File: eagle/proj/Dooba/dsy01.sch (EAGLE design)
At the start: 75 parts, among them P1 DIO, P10 SWD_CORE(SWCLK-SWDIO-GND), P11 SWD_CORE(SWCLK-SWDIO-GND), P2 CKI-CKO, P3 NOT, P4 RDY, P5 PWR(VIN-GND-RST), P6 SWD_CORE(SWCLK-SWDIO-GND), P7 SWD_CORE(SWCLK-SWDIO-GND), P8 SWD_CORE(SWCLK-SWDIO-GND), P9 SWD_CORE(SWCLK-SWDIO-GND), U1 STM32F071LQFP100, U10 S25FLXXXSSOIC16, U2 AS6C1608TSOPII-44, U3 STM32F030LQFP32, U5 STM32F030LQFP32, U6 STM32F030LQFP32, U7 STM32F030LQFP32, U8 MIC550XSOT23, U9 STM32F030LQFP32, X1 8MHz, X2 8MHz, X4 8MHz, X5 8MHz, X6 8MHz, X7 8MHz

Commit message: Finished routing DSY01 Added LEDs on DSY01
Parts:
- added D1, D2, D3, D4, D5, D6: LED0805, dooba:LED0805
- added R1, R2, R3, R4, R5, R6: 330, dooba:RES0805
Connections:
- new net N$109: R5.2, U9.PA15
- new net N$110: D6.1, R6.1
- new net N$111: R6.2, U1.PF9
- new net N$54: D1.1, R1.1
- new net N$56: R1.2, U3.PA15
- new net N$62: D2.1, R2.1
- new net N$70: R2.2, U5.PA15
- new net N$74: D3.1, R3.1
- new net N$87: R3.2, U6.PA15
- new net N$88: D4.1, R4.1
- new net N$89: R4.2, U7.PA15
- new net N$92: D5.1, R5.1
- net GND: now also D1.2, D2.2, D3.2, D4.2, D5.2, D6.2; no longer U1.PF9, U3.PA15, U5.PA15, U6.PA15, U7.PA15, U9.PA15

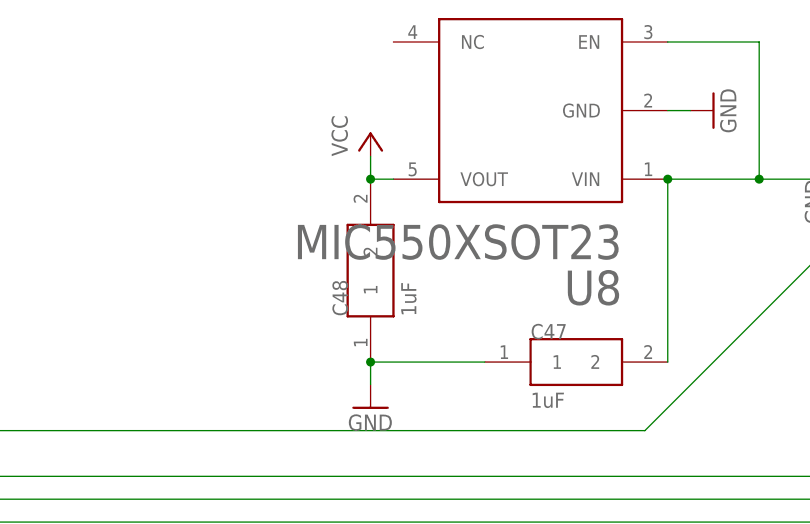
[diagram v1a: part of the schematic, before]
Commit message: Added more decorations to DSY01
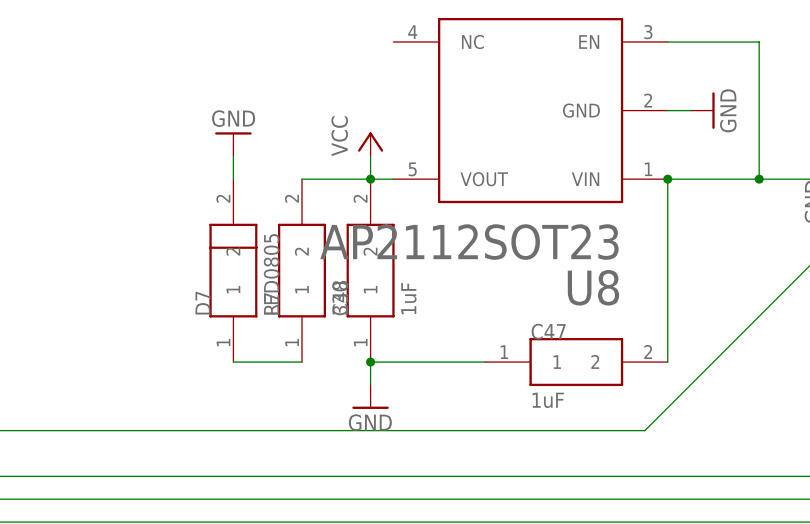
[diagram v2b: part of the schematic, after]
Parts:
- added D7: LED0805, dooba:LED0805
- added R7: 330, dooba:RES0805
- U8: value MIC550XSOT23 -> AP2112SOT23; device dooba:MIC550XSOT23 -> dooba:AP2112SOT23
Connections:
- new net N$112: D7.1, R7.1
- net GND: now also D7.2
- net VCC: now also R7.2
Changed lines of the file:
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@@
 <part name="C46" library="dooba" deviceset="CAP" device="0805" value="27pF"/>
 <part name="GND37" library="supply1" deviceset="GND" device=""/>
-<part name="U8" library="dooba" deviceset="MIC550X" device="SOT23"/>
+<part name="U8" library="dooba" deviceset="AP2112" device="SOT23"/>
 <part name="C47" library="dooba" deviceset="CAP" device="0805" value="1uF"/>
 <part name="C48" library="dooba" deviceset="CAP" device="0805" value="1uF"/>
@@
 <part name="R6" library="dooba" deviceset="RES" device="0805" value="330"/>
 <part name="GND49" library="supply1" deviceset="GND" device=""/>
+<part name="D7" library="dooba" deviceset="LED" device="0805"/>
+<part name="R7" library="dooba" deviceset="RES" device="0805" value="330"/>
+<part name="GND61" library="supply1" deviceset="GND" device=""/>
 </parts>
 <sheets>
@@
 <instance part="R6" gate="R1" x="381" y="416.56"/>
 <instance part="GND49" gate="1" x="396.24" y="424.18" rot="R90"/>
+<instance part="D7" gate="D1" x="1534.16" y="1120.14" rot="R90"/>
+<instance part="R7" gate="R1" x="1541.78" y="1120.14" rot="R90"/>
+<instance part="GND61" gate="1" x="1534.16" y="1135.38" rot="R180"/>
 </instances>
 <busses>
@@
 <wire x1="429.26" y1="401.32" x2="431.8" y2="401.32" width="0.1524" layer="91"/>
 </segment>
+<segment>
+<pinref part="D7" gate="D1" pin="2"/>
+<pinref part="GND61" gate="1" pin="GND"/>
+<wire x1="1534.16" y1="1130.3" x2="1534.16" y2="1132.84" width="0.1524" layer="91"/>
+</segment>
 </net>
 <net name="VCC" class="0">
@@
 <wire x1="1549.4" y1="1130.3" x2="1551.94" y2="1130.3" width="0.1524" layer="91"/>
 <junction x="1549.4" y="1130.3"/>
+<pinref part="R7" gate="R1" pin="2"/>
+<wire x1="1549.4" y1="1130.3" x2="1541.78" y2="1130.3" width="0.1524" layer="91"/>
 </segment>
 <segment>
@@
 </segment>
 </net>
+<net name="N$112" class="0">
+<segment>
+<pinref part="R7" gate="R1" pin="1"/>
+<pinref part="D7" gate="D1" pin="1"/>
+<wire x1="1541.78" y1="1109.98" x2="1534.16" y2="1109.98" width="0.1524" layer="91"/>
+</segment>
+</net>
